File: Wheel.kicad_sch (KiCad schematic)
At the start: 44 parts, among them J1 USB_C_Receptacle_USB2.0_16P, J5 Conn_01x06, J6 Conn_01x03, J7 Conn_01x05, SW1 SW_Push, SW2 SW_Push, U1 STM32F407VGTx, U2 AMS1117-3.3

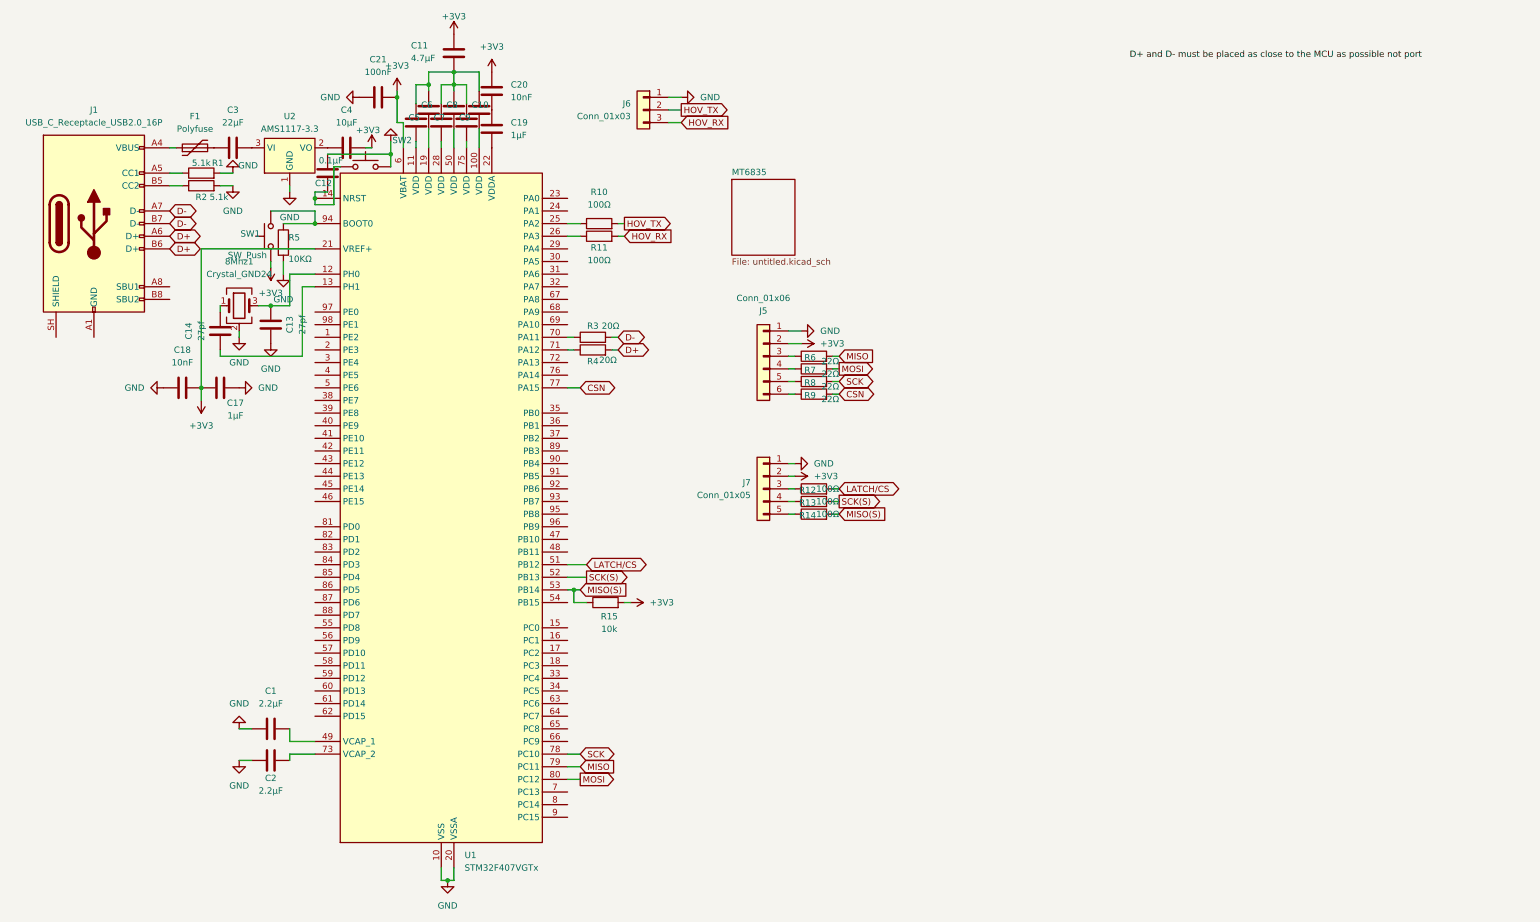
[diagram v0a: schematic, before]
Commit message: Update
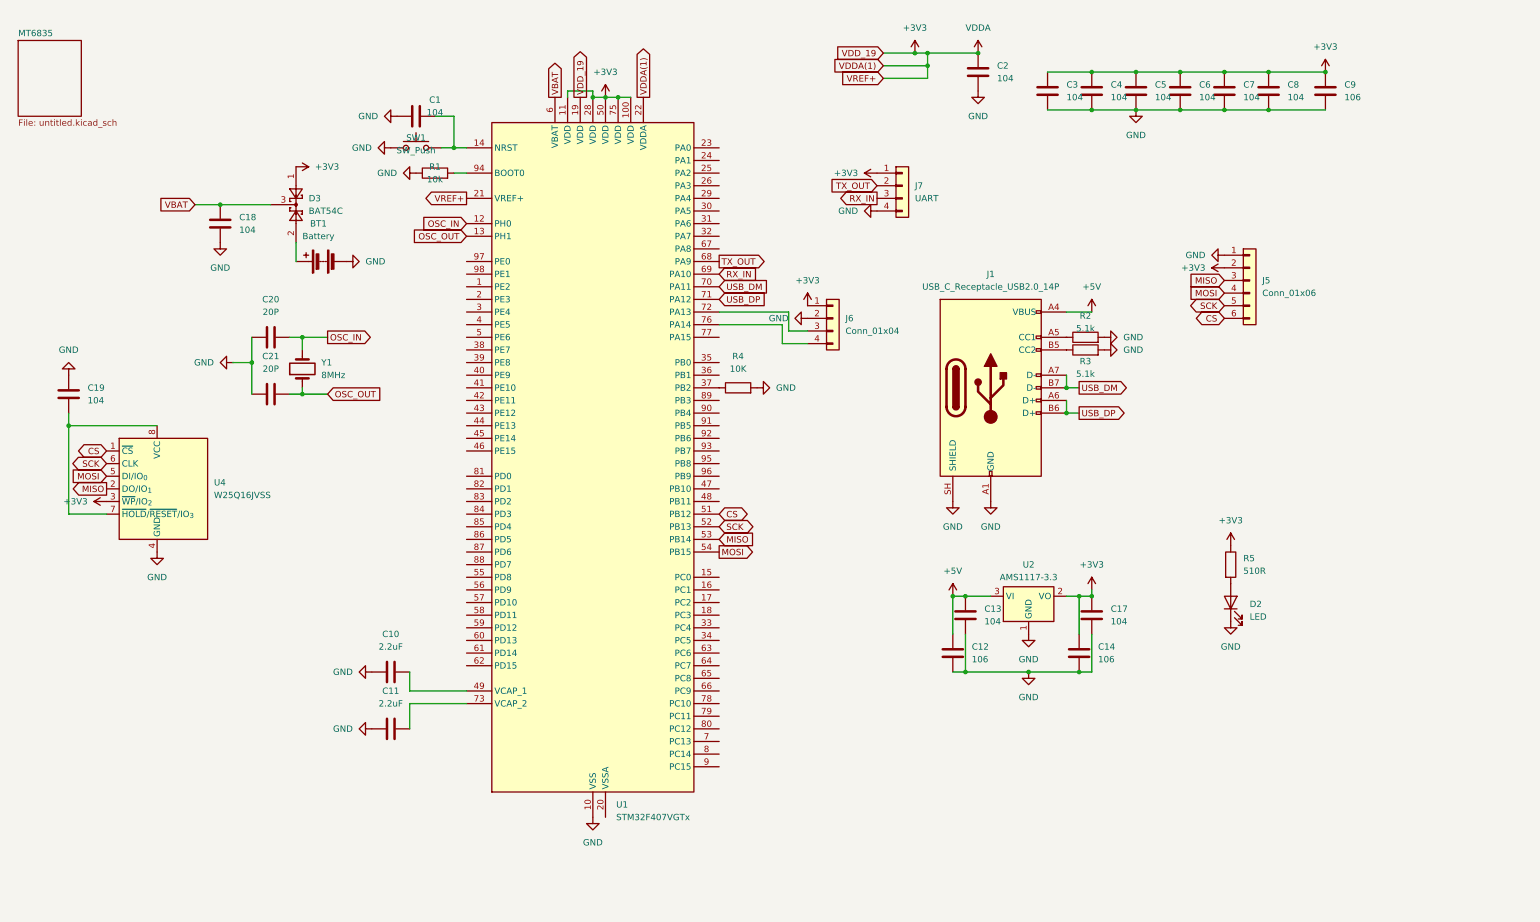
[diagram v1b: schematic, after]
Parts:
- removed 8Mhz1: Crystal_GND24, Crystal:Crystal_SMD_3225-4Pin_3.2x2.5mm, symbol Device:Crystal_GND24
- removed F1: Polyfuse, Fuse:Fuse_1812_4532Metric, symbol Device:Polyfuse
- removed J1: USB_C_Receptacle_USB2.0_16P, Connector_USB:USB_C_Receptacle_HRO_TYPE-C-31-M-12, symbol Connector:USB_C_Receptacle_USB2.0_16P
- removed J6: Conn_01x03, Connector_PinHeader_2.54mm:PinHeader_1x03_P2.54mm_Vertical, symbol Connector_Generic:Conn_01x03
- removed J7: Conn_01x05, Connector_PinHeader_2.54mm:PinHeader_1x05_P2.54mm_Vertical, symbol Connector_Generic:Conn_01x05
- removed R10, R11, R12, R13, R14: 100Ω, Resistor_SMD:R_0402_1005Metric, symbol Device:R
- removed R15: 10k, Resistor_SMD:R_0402_1005Metric, symbol Device:R
- removed R6, R7, R8, R9: 22Ω, Resistor_SMD:R_0402_1005Metric, symbol Device:R
- removed SW2: SW_Push, Button_Switch_SMD:SW_Push_SPST_NO_Alps_SKRK, symbol Switch:SW_Push
- added BT1: Battery, Battery:BatteryHolder_Keystone_3002_1x2032, symbol Device:Battery
- added D2: LED, LED_SMD:LED_0603_1608Metric, symbol Device:LED
- added D3: BAT54C, Package_TO_SOT_SMD:SOT-23, symbol Diode:BAT54C
- added J1: USB_C_Receptacle_USB2.0_14P, Connector_USB:USB_C_Receptacle_HRO_TYPE-C-31-M-12, symbol Connector:USB_C_Receptacle_USB2.0_14P
- added J6: Conn_01x04, Connector:FanPinHeader_1x04_P2.54mm_Vertical, symbol Connector_Generic:Conn_01x04
- added J7: UART, Connector:FanPinHeader_1x04_P2.54mm_Vertical, symbol Connector_Generic:Conn_01x04
- added U4: W25Q16JVSS, Package_SO:SOIC-8_5.3x5.3mm_P1.27mm, symbol Memory_Flash:W25Q16JVSS
- added Y1: 8MHz, Crystal:Crystal_SMD_5032-2Pin_5.0x3.2mm, symbol Device:Crystal
- C1, C2: value 2.2µF -> 104; footprint Capacitor_SMD:C_0402_1005Metric -> Capacitor_SMD:C_0603_1608Metric
- C10: value 100nF -> 2.2uF; footprint Capacitor_SMD:C_0402_1005Metric -> Capacitor_SMD:C_0603_1608Metric
- C11: value 4.7µF -> 2.2uF; footprint Capacitor_SMD:C_0402_1005Metric -> Capacitor_SMD:C_0603_1608Metric
- C12: value 0.1µF -> 106; footprint Capacitor_SMD:C_0402_1005Metric -> Capacitor_SMD:C_0805_2012Metric
- C13: value 27pf -> 104; footprint Capacitor_SMD:C_0402_1005Metric -> Capacitor_SMD:C_0603_1608Metric
- C14: value 27pf -> 106; footprint Capacitor_SMD:C_0402_1005Metric -> Capacitor_SMD:C_0805_2012Metric
- C17, C19: value 1µF -> 104; footprint Capacitor_SMD:C_0402_1005Metric -> Capacitor_SMD:C_0603_1608Metric
- C18: value 10nF -> 104; footprint Capacitor_SMD:C_0402_1005Metric -> Capacitor_SMD:C_0603_1608Metric
- C20: value 10nF -> 20P; footprint Capacitor_SMD:C_0402_1005Metric -> Capacitor_SMD:C_0603_1608Metric
- C21: value 100nF -> 20P; footprint Capacitor_SMD:C_0402_1005Metric -> Capacitor_SMD:C_0603_1608Metric
- C3: value 22µF -> 104; footprint Capacitor_SMD:C_0805_2012Metric -> Capacitor_SMD:C_0603_1608Metric
- C4: value 10µF -> 104; footprint Capacitor_SMD:C_0805_2012Metric -> Capacitor_SMD:C_0603_1608Metric
- C5, C6, C7, C8: value 100nF -> 104; footprint Capacitor_SMD:C_0402_1005Metric -> Capacitor_SMD:C_0603_1608Metric
- C9: value 100nF -> 106; footprint Capacitor_SMD:C_0402_1005Metric -> Capacitor_SMD:C_0805_2012Metric
- R1: value 5.1k -> 10k; footprint Resistor_SMD:R_0402_1005Metric -> Resistor_SMD:R_0603_1608Metric
- R2: footprint Resistor_SMD:R_0402_1005Metric -> Resistor_SMD:R_0603_1608Metric
- R3: value 20Ω -> 5.1k; footprint Resistor_SMD:R_0402_1005Metric -> Resistor_SMD:R_0603_1608Metric
- R4: value 20Ω -> 10K; footprint Resistor_SMD:R_0402_1005Metric -> Resistor_SMD:R_0603_1608Metric
- R5: value 10KΩ -> 510R; footprint Resistor_SMD:R_0402_1005Metric -> Resistor_SMD:R_0603_1608Metric
- SW1: footprint Button_Switch_SMD:SW_Push_SPST_NO_Alps_SKRK -> Button_Switch_SMD:SW_SPST_FSMSM
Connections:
- net D+ is gone; now on net GND: R4.2
- net D- is gone; now on net GND: R3.2
- net LATCH/CS is gone; now on net CS: U1.51 (PB12)
- net MISO(S) is gone; now on net MISO: U1.53 (PB14)
- net SCK(S) is gone; now on net SCK: U1.52 (PB13)
- net +3V3: now also C14.1, C2.2, C3.1, C4.1, C5.1, C6.1, C7.1, C8.1, C9.1, R5.1, U1.100 (VDD), U1.11 (VDD), U1.19 (VDD), U1.22 (VDDA), U1.28 (VDD), U1.50 (VDD), U1.75 (VDD), U2.2 (VO), D3.1, J6.1 (Pin_1), J7.1 (Pin_1), U4.3 (~{WP}/IO_{2}); no longer C11.1, C18.2, C20.1, C21.2, C4.2, SW1.1, U1.6 (VBAT)
- net GND: now also C10.1, C11.1, C12.2, C13.2, C14.2, C18.2, C19.1, C20.1, C3.2, C4.2, C5.2, C6.2, C7.2, C8.2, C9.2, R1.1, SW1.1, BT1.2 (-), D2.1 (K), J1.A1 (GND), J1.A12 (GND), J1.B1 (GND), J1.B12 (GND), J1.SH (SHIELD), J6.2 (Pin_2), J7.4 (Pin_4), U4.4 (GND); no longer C12.1, C13.1, C18.1, R1.2, R5.2, U1.20 (VSSA)
- net MISO: now also J5.3 (Pin_3), U4.2 (DO/IO_{1}); no longer U1.79 (PC11)
- net MOSI: now also J5.4 (Pin_4), U1.54 (PB15), U4.5 (DI/IO_{0}); no longer U1.80 (PC12)
- net SCK: now also J5.5 (Pin_5), U4.6 (CLK); no longer U1.78 (PC10)
- net at R3.1: now also J1.B5 (CC2); no longer U1.70 (PA11)
- net OSC_IN: now reaches C20.2
- net OSC_IN: now also U1.12 (PH0), Y1.2; no longer C19.1
- net CS: now reaches J5.6 (Pin_6)
- net CS: now also U4.1 (~{CS})
- net +5V: now reaches U2.3 (VI)
- net +5V: now also C12.1, C13.1, J1.A4 (VBUS), J1.A9 (VBUS), J1.B4 (VBUS), J1.B9 (VBUS); no longer C3.2
- net at C19.2: now also U4.7 (~{HOLD}/~{RESET}/IO_{3}), U4.8 (VCC); no longer U1.22 (VDDA)
- net OSC_OUT: now reaches U1.13 (PH1)
- net OSC_OUT: now also C21.2, Y1.1; no longer C14.1
- net at U1.14 (NRST): now also C1.2, SW1.2; no longer C12.2
- net at R2.1: now also J1.A5 (CC1)
- net at C10.2: now also U1.49 (VCAP_1); no longer U1.100 (VDD)
- net at U1.37 (PB2): now also R4.1
- net TX_OUT: now reaches U1.68 (PA9)
- net TX_OUT: now also J7.2 (Pin_2)
- net RX_IN: now reaches U1.69 (PA10)
- net RX_IN: now also J7.3 (Pin_3)
- net USB_DP: now reaches U1.71 (PA12)
- net USB_DP: now also J1.A6 (D+), J1.B6 (D+); no longer R4.1
- net at U1.72 (PA13): now also J6.3 (Pin_3)
- net at U1.73 (VCAP_2): now also C11.2; no longer C2.2
- net at U1.76 (PA14): now also J6.4 (Pin_4)
- net CSN: no longer names the net of U1.77 (PA15)
- new net: BT1.1 (+), D3.2
- new net: R1.2, U1.94 (BOOT0)
- new net: D2.2 (A), R5.2
- new net USB_DM: J1.A7 (D-), J1.B7 (D-), U1.70 (PA11)
- new net VBAT: C18.1, D3.3, U1.6 (VBAT)
